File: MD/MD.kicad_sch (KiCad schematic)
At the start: 75 parts, among them J1 Conn_01x05_Pin, J2 Conn_01x05_Pin, J3 Conn_02x07_Odd_Even, J4 Conn_01x06_Pin, Q1 2SA1015, Q2 μPA2753GR, Q3 BSS138, Q4 BSS138, Q5 μPA2753GR, SW1 SW_Push, SW2 SW_DIP_x04, SW3 SW_SPDT, U1 AZ1117-3.3, U2 MAX3485, U3 STM32C011F4Px, U4 IR2302, U5 IR2302, X1 MEMS_Oscillator_SiT2001B

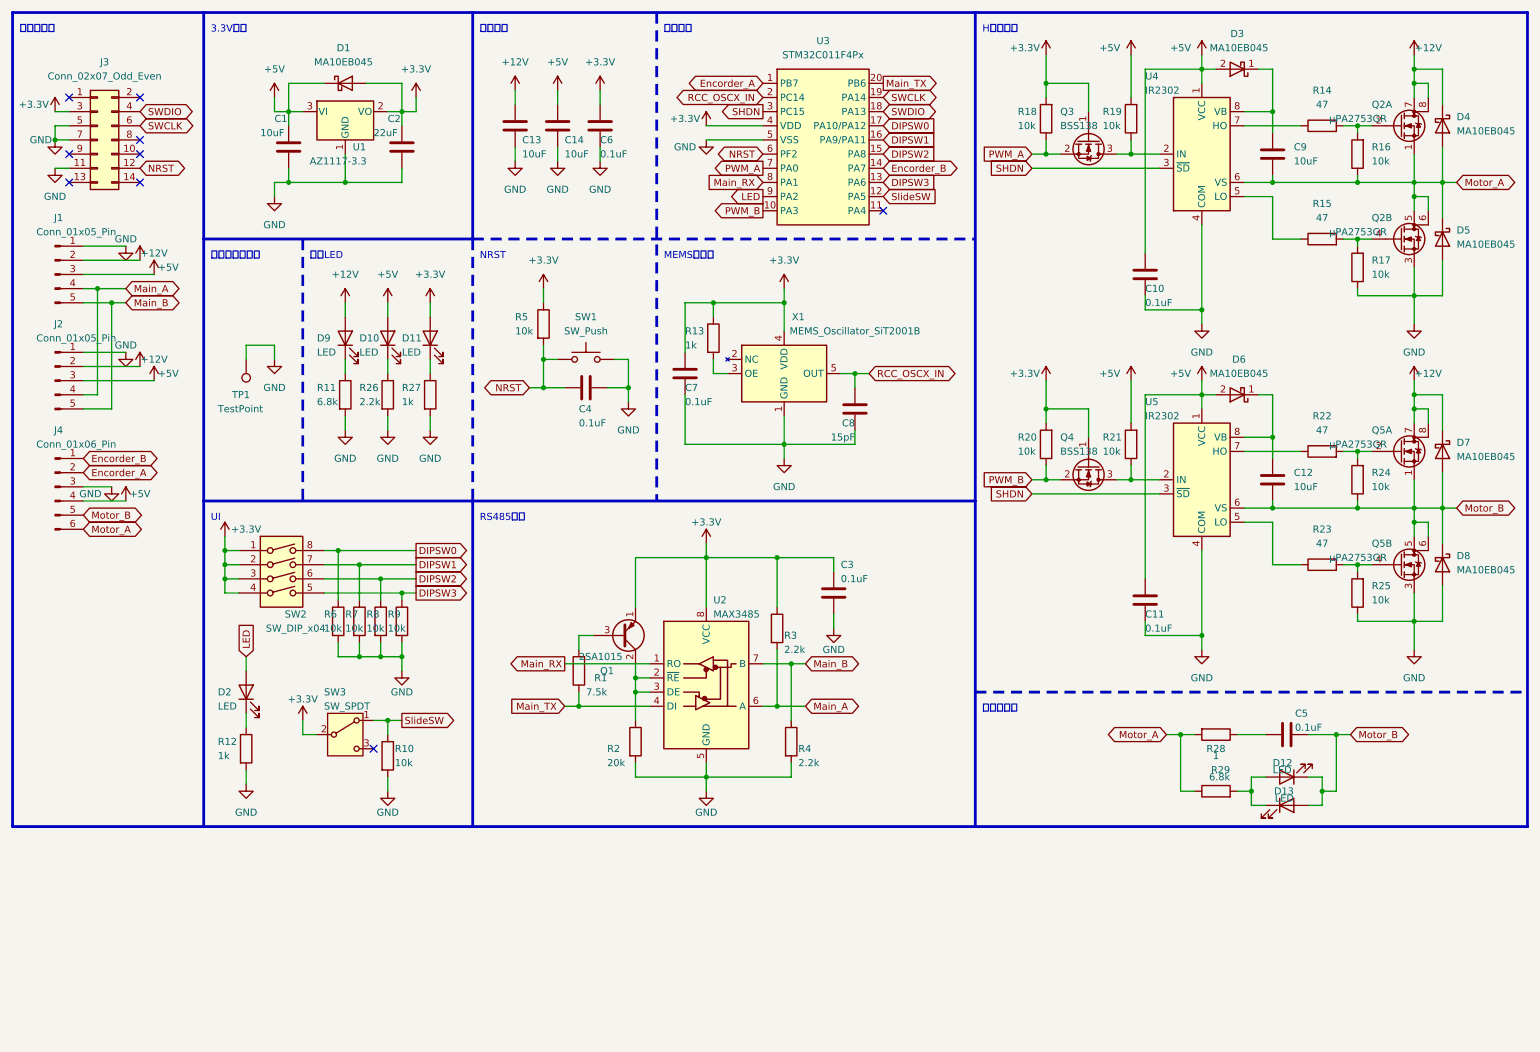
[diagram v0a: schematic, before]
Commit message: 回路図完成
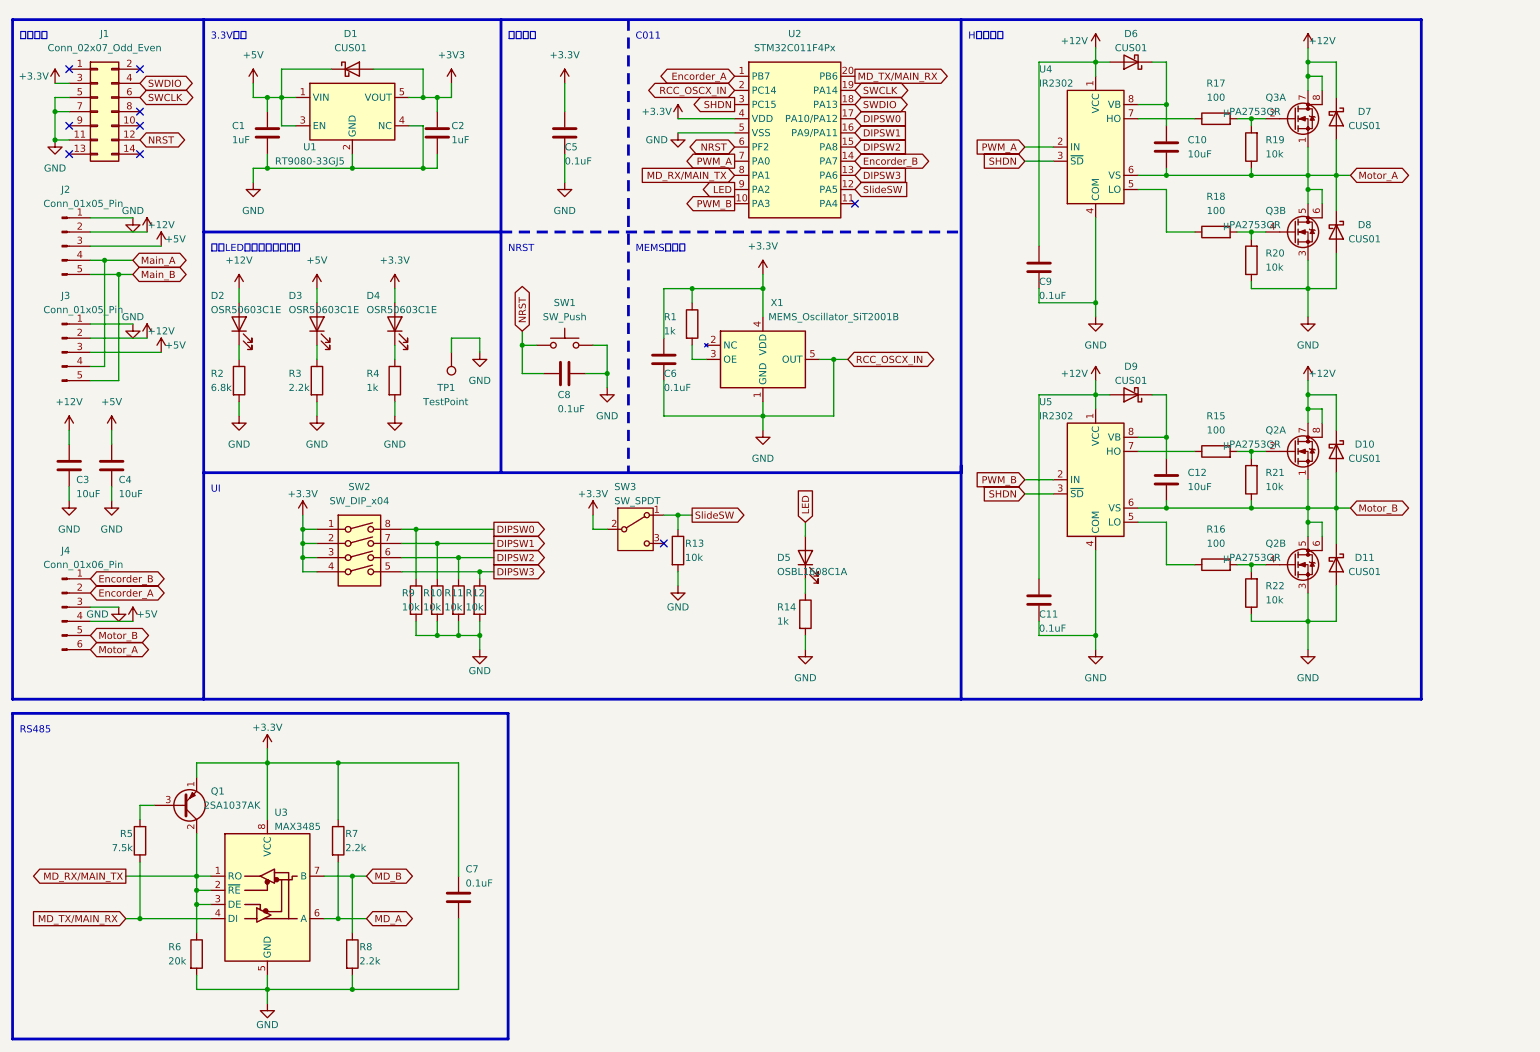
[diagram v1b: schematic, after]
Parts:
- removed C13, C14: 10uF, Capacitor_SMD:C_0603_1608Metric_Pad1.08x0.95mm_HandSolder, symbol Device:C
- removed D10, D11, D12, D13, D9: LED, LED_SMD:LED_0603_1608Metric_Pad1.05x0.95mm_HandSolder, symbol Device:LED
- removed D3, D4, D5: MA10EB045, Diode_SMD:Vishay_SMPA, symbol Device:D_Schottky
- removed J1: Conn_01x05_Pin, Connector_JST:JST_XH_B5B-XH-A_1x05_P2.50mm_Vertical, symbol Connector:Conn_01x05_Pin
- removed J3: Conn_02x07_Odd_Even, Tomoshibi_Library:BoxHeader_2x07_P1.27mm_Horizontal, symbol Connector_Generic:Conn_02x07_Odd_Even
- removed Q3, Q4: BSS138, Package_TO_SOT_SMD:SOT-23, symbol Transistor_FET:BSS138
- removed Q5: μPA2753GR, Package_SO:SOP-8_3.9x4.9mm_P1.27mm, symbol Device:Q_Dual_NMOS_S1G1S2G2D2D2D1D1
- removed R23: 47, Resistor_SMD:R_0603_1608Metric_Pad0.98x0.95mm_HandSolder, symbol Device:R
- removed R24, R25: 10k, Resistor_SMD:R_0603_1608Metric_Pad0.98x0.95mm_HandSolder, symbol Device:R
- removed R26: 2.2k, Resistor_SMD:R_0603_1608Metric_Pad0.98x0.95mm_HandSolder, symbol Device:R
- removed R27: 1k, Resistor_SMD:R_0603_1608Metric_Pad0.98x0.95mm_HandSolder, symbol Device:R
- removed R28: 1, Resistor_SMD:R_0603_1608Metric_Pad0.98x0.95mm_HandSolder, symbol Device:R
- removed R29: 6.8k, Resistor_SMD:R_0603_1608Metric_Pad0.98x0.95mm_HandSolder, symbol Device:R
- removed U1: AZ1117-3.3, Package_TO_SOT_SMD:SOT-223-3_TabPin2, symbol Regulator_Linear:AZ1117-3.3
- removed U2: MAX3485, Package_SO:SOP-8_3.76x4.96mm_P1.27mm, symbol Interface_UART:MAX3485
- removed U3: STM32C011F4Px, Package_SO:SSOP-20_4.4x6.5mm_P0.65mm, symbol Tomoshibi_Library:STM32C011F4Px
- added D10, D11, D9: CUS01, Diode_SMD:D_SOD-323_HandSoldering, symbol Device:D_Schottky
- added D3, D4: OSR50603C1E, LED_SMD:LED_0603_1608Metric_Pad1.05x0.95mm_HandSolder, symbol Device:LED
- added D5: OSBL1608C1A, LED_SMD:LED_0603_1608Metric_Pad1.05x0.95mm_HandSolder, symbol Device:LED
- added J1: Conn_02x07_Odd_Even, Tomoshibi_Library:BoxHeader_2x07_P1.27mm_Horizontal, symbol Connector_Generic:Conn_02x07_Odd_Even
- added J3: Conn_01x05_Pin, Connector_JST:JST_XH_B5B-XH-A_1x05_P2.50mm_Vertical, symbol Connector:Conn_01x05_Pin
- added Q3: μPA2753GR, Package_SO:SOP-8_3.9x4.9mm_P1.27mm, symbol Device:Q_Dual_NMOS_S1G1S2G2D2D2D1D1
- added U1: RT9080-33GJ5, Package_TO_SOT_SMD:TSOT-23-5, symbol Tomoshibi_Library:RT9080-33GJ5
- added U2: STM32C011F4Px, Package_SO:TSSOP-20_4.4x6.5mm_P0.65mm, symbol Tomoshibi_Library:STM32C011F4Px
- added U3: MAX3485, Package_SO:SOP-8_3.76x4.96mm_P1.27mm, symbol Interface_UART:MAX3485
- C1: value 10uF -> 1uF
- C10, C3, C4: value 0.1uF -> 10uF
- C2: value 22uF -> 1uF; footprint Capacitor_SMD:C_0805_2012Metric_Pad1.18x1.45mm_HandSolder -> Capacitor_SMD:C_0603_1608Metric_Pad1.08x0.95mm_HandSolder
- C8: value 15pF -> 0.1uF
- C9: value 10uF -> 0.1uF
- D1, D6, D7, D8: value MA10EB045 -> CUS01; footprint Diode_SMD:Vishay_SMPA -> Diode_SMD:D_SOD-323_HandSoldering
- D2: value LED -> OSR50603C1E
- Q1: value 2SA1015 -> 2SA1037AK; footprint Package_TO_SOT_THT:TO-92_Inline -> Package_TO_SOT_SMD:SOT-23-3
- R1: value 7.5k -> 1k
- R11: value 6.8k -> 10k
- R12, R13: value 1k -> 10k
- R14: value 47 -> 1k
- R15: value 47 -> 100
- R16, R17, R18: value 10k -> 100
- R2: value 20k -> 6.8k
- R22: value 47 -> 10k
- R4: value 2.2k -> 1k
- R5: value 10k -> 7.5k
- R6: value 10k -> 20k
- R7, R8: value 10k -> 2.2k
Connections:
- net Main_TX is gone; now on net +3.3V: R1.1
- net +12V: now also C11.1, C3.1, C9.1, D2.2 (A), D6.2 (A), U4.1 (VCC), U5.1 (VCC), D10.1 (K), D9.2 (A), J3.2 (Pin_2), Q3.7 (D), Q3.8 (D)
- net +3.3V: now also C5.1, R7.1, D4.2 (A), J1.3 (Pin_3), U2.4 (VDD), U3.8 (VCC); no longer C2.1, C3.1, D1.2 (A), R13.1, R18.2, R20.2, R3.1, R5.1
- net +5V: now also C4.1, D3.2 (A), J3.3 (Pin_3), U1.1 (VIN), U1.3 (EN); no longer C10.1, C11.1, D6.2 (A), R19.2, R21.2, U4.1 (VCC), U5.1 (VCC)
- net DIPSW0: now also R9.1, U2.17 (PA10/PA12); no longer R6.1
- net DIPSW1: now also R10.1, U2.16 (PA9/PA11); no longer R7.1
- net DIPSW2: now also R11.1, U2.15 (PA8); no longer R8.1
- net DIPSW3: now also R12.1, U2.13 (PA6); no longer R9.1
- net Encorder_A: now also U2.1 (PB7)
- net Encorder_B: now also U2.14 (PA7)
- net GND: now also C4.2, C5.2, C9.2, R13.2, R14.2, R20.1, R22.1, R3.2, X1.5 (OUT), D11.2 (A), J1.11 (Pin_11), J1.5 (Pin_5), J1.7 (Pin_7), J3.1 (Pin_1), Q3.3 (S), U1.2 (GND), U1.4 (NC), U2.2 (PC14), U2.5 (VSS), U3.5 (GND); no longer C10.2, C4.1, R17.1, R7.2
- net LED: now also D5.2 (A), U2.9 (PA2); no longer D2.2 (A)
- net Main_A: now also J3.4 (Pin_4); no longer R3.2
- net Main_B: now also J3.5 (Pin_5); no longer R4.1
- net Motor_A: now also C10.2, D7.2 (A), D8.1 (K), R19.1, Q3.1 (S), Q3.5 (D), Q3.6 (D); no longer C9.2, Q2.1 (S), Q2.5 (D), Q2.6 (D), R16.1
- net Motor_B: now also Q2.1 (S), Q2.5 (D), Q2.6 (D), R21.1, D10.2 (A), D11.1 (K); no longer C5.2, D7.2 (A), D8.1 (K)
- net NRST: now also C8.2, J1.12 (Pin_12), U2.6 (PF2); no longer C4.2, R5.2
- net PWM_A: now also U4.2 (IN), U2.7 (PA0); no longer R18.1
- net PWM_B: now also U5.2 (IN), U2.10 (PA3); no longer R20.1
- net SHDN: now also U2.3 (PC15)
- net SWCLK: now also J1.6 (Pin_6), U2.19 (PA14)
- net SWDIO: now also J1.4 (Pin_4), U2.18 (PA13)
- net SlideSW: now also R13.1, U2.12 (PA5); no longer R10.1
- net at X1.3 (OE): now also R1.2; no longer R13.2
- net at U5.5 (LO): now also R16.1
- net at U5.7 (HO): now also R15.1; no longer R22.1
- net at C12.1, U5.8 (VB): now also D9.1 (K); no longer D6.1 (K)
- net at Q1.3 (B): now also R5.2; no longer R1.2
- net at U4.5 (LO): now also R18.1; no longer R15.1
- net at R14.1: now also D5.1 (K); no longer U4.7 (HO)
- net at U4.8 (VB): now also C10.1, D6.1 (K); no longer C9.1
- net at R2.1: now also D2.1 (K); no longer Q1.2 (C)
- net at R22.2: now also Q2.4 (G), R16.2
- removed net RCC_OSCX_IN: C8.2, X1.5 (OUT)
- new net: D4.1 (K), R4.1
- new net: R17.1, U4.7 (HO)
- new net: Q3.2 (G), R17.2, R19.2
- new net: D3.1 (K), R3.1
- new net: Q3.4 (G), R18.2, R20.2
- new net: Q2.2 (G), R15.2, R21.2
- new net +3V3: C2.1, D1.2 (A), U1.5 (VOUT)
- new net MD_A: R7.2, U3.6 (A)
- new net MD_B: R8.1, U3.7 (B)
- new net MD_RX/MAIN_TX: Q1.2 (C), R6.1, U2.8 (PA1), U3.1 (RO), U3.2 (~{RE}), U3.3 (DE)
- new net MD_TX/MAIN_RX: R5.1, U2.20 (PB6), U3.4 (DI)
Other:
- note added: "C011"
- note added: "RS485"
- note added: "コネクタ"
- note added: "電源LED・テストポイント"
- note removed: "RS485変換"
- note removed: "コネクター"
- note removed: "スナバ回路"
- note removed: "テストポイント"
- note removed: "マイコン"
- note removed: "電源LED"
